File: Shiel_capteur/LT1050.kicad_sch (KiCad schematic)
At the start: 22 parts, among them P1 Power, P2 Analog, P3 Digital, P4 Digital, P5 CONN_01X01, P6 CONN_01X01, P7 CONN_01X01, P8 CONN_01X01, U0 Capteur_graphite, U1 LT1050, U2 Module_bluetooth, U3 OLED

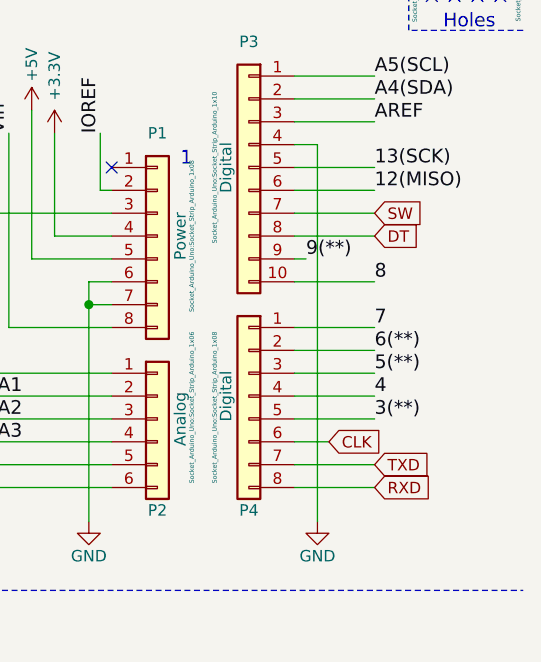
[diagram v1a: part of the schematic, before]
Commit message: mise à jour pcb
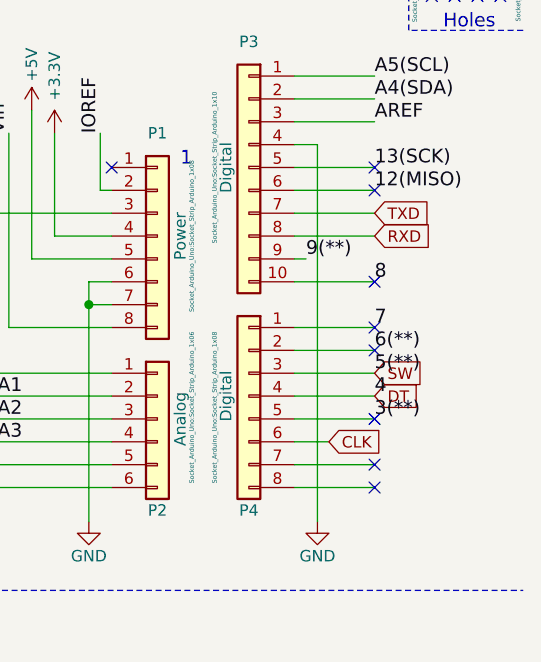
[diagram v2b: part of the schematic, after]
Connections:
- net 4 is gone; now on net DT: P4.4 (Pin_4)
- net 5(**) is gone; now on net SW: P4.3 (Pin_3)
- net DT: no longer P3.8 (Pin_8)
- net RXD: now also P3.8 (Pin_8); no longer P4.8 (Pin_8)
- net SW: no longer P3.7 (Pin_7)
- net TXD: now also P3.7 (Pin_7); no longer P4.7 (Pin_7)
- no-connect marks 9 -> 17
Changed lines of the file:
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@@
   (no_connect (at 274.32 21.59))
   (no_connect (at 146.05 48.26))
+  (no_connect (at 267.97 40.64))
+  (no_connect (at 267.97 43.18))
+  (no_connect (at 267.97 73.66))
+  (no_connect (at 267.97 76.2))
+  (no_connect (at 267.97 68.58))
+  (no_connect (at 267.97 58.42))
+  (no_connect (at 267.97 60.96))
+  (no_connect (at 267.97 53.34))
   (no_connect (at 113.03 151.13))
   (no_connect (at 276.86 21.59))
@@
     )
   )
+  (global_label "RXD" (shape input) (at 267.97 48.26 0) (fields_autoplaced)
+    (effects (font (size 1.27 1.27)) (justify left))
+    (property "Intersheet References" "${INTERSHEET_REFS}" (id 0) (at 274.3231 48.1806 0)
+      (effects (font (size 1.27 1.27)) (justify left) hide)
+    )
+  )
   (global_label "IN-" (shape input) (at 185.42 43.18 0) (fields_autoplaced)
     (effects (font (size 1.27 1.27)) (justify left))
     (property "Intersheet References" "${INTERSHEET_REFS}" (id 0) (at 191.5312 43.1006 0)
-      (effects (font (size 1.27 1.27)) (justify left) hide)
-    )
-  )
-  (global_label "DT" (shape input) (at 267.97 48.26 0) (fields_autoplaced)
-    (effects (font (size 1.27 1.27)) (justify left))
-    (property "Intersheet References" "${INTERSHEET_REFS}" (id 0) (at 272.8112 48.1806 0)
       (effects (font (size 1.27 1.27)) (justify left) hide)
     )
@@
     )
   )
-  (global_label "RXD" (shape input) (at 267.97 76.2 0) (fields_autoplaced)
-    (effects (font (size 1.27 1.27)) (justify left))
-    (property "Intersheet References" "${INTERSHEET_REFS}" (id 0) (at 274.3231 76.1206 0)
+  (global_label "CLK" (shape input) (at 262.89 71.12 0) (fields_autoplaced)
+    (effects (font (size 1.27 1.27)) (justify left))
+    (property "Intersheet References" "${INTERSHEET_REFS}" (id 0) (at 269.0617 71.0406 0)
       (effects (font (size 1.27 1.27)) (justify left) hide)
     )
@@
     (effects (font (size 1.27 1.27)) (justify left))
     (property "Intersheet References" "${INTERSHEET_REFS}" (id 0) (at 98.8212 65.9606 0)
+      (effects (font (size 1.27 1.27)) (justify left) hide)
+    )
+  )
+  (global_label "DT" (shape input) (at 267.97 66.04 0) (fields_autoplaced)
+    (effects (font (size 1.27 1.27)) (justify left))
+    (property "Intersheet References" "${INTERSHEET_REFS}" (id 0) (at 272.8112 65.9606 0)
       (effects (font (size 1.27 1.27)) (justify left) hide)
     )
@@
     )
   )
-  (global_label "TXD" (shape input) (at 267.97 73.66 0) (fields_autoplaced)
-    (effects (font (size 1.27 1.27)) (justify left))
-    (property "Intersheet References" "${INTERSHEET_REFS}" (id 0) (at 274.0207 73.5806 0)
-      (effects (font (size 1.27 1.27)) (justify left) hide)
-    )
-  )
-  (global_label "SW" (shape input) (at 267.97 45.72 0) (fields_autoplaced)
-    (effects (font (size 1.27 1.27)) (justify left))
-    (property "Intersheet References" "${INTERSHEET_REFS}" (id 0) (at 273.2346 45.6406 0)
+  (global_label "SW" (shape input) (at 267.97 63.5 0) (fields_autoplaced)
+    (effects (font (size 1.27 1.27)) (justify left))
+    (property "Intersheet References" "${INTERSHEET_REFS}" (id 0) (at 273.2346 63.4206 0)
+      (effects (font (size 1.27 1.27)) (justify left) hide)
+    )
+  )
+  (global_label "TXD" (shape input) (at 267.97 45.72 0) (fields_autoplaced)
+    (effects (font (size 1.27 1.27)) (justify left))
+    (property "Intersheet References" "${INTERSHEET_REFS}" (id 0) (at 274.0207 45.6406 0)
       (effects (font (size 1.27 1.27)) (justify left) hide)
     )
@@
     )
   )
-  (global_label "CLK" (shape input) (at 262.89 71.12 0) (fields_autoplaced)
-    (effects (font (size 1.27 1.27)) (justify left))
-    (property "Intersheet References" "${INTERSHEET_REFS}" (id 0) (at 269.0617 71.0406 0)
-      (effects (font (size 1.27 1.27)) (justify left) hide)
-    )
-  )
